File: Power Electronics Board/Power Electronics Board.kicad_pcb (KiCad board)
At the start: 2 copper layers, 137.7 x 71.1 mm, 69 parts, among them J1 Conn_01x02, J2 Conn_01x02, J3 1054301102, J4 1054301102, J5 1054311102, J6 Conn_01x02, J7 1054301108, K2 AZ2150-1A-12DEF, K3 EW60-1A3-CL12D04,00000, K4 DS1E-ML-DC12V, Q1 AO3400A, Q2 AO3400A, Q3 DMG2301L, U1 MCP6004, U3 MCP1703AT-5002E/CB, U4 CC1R5-1205SR-E, U5 ISOM8111DFSR, U6 MCP6004, U7 LM555xM, U8 SZNUD3124LT1G

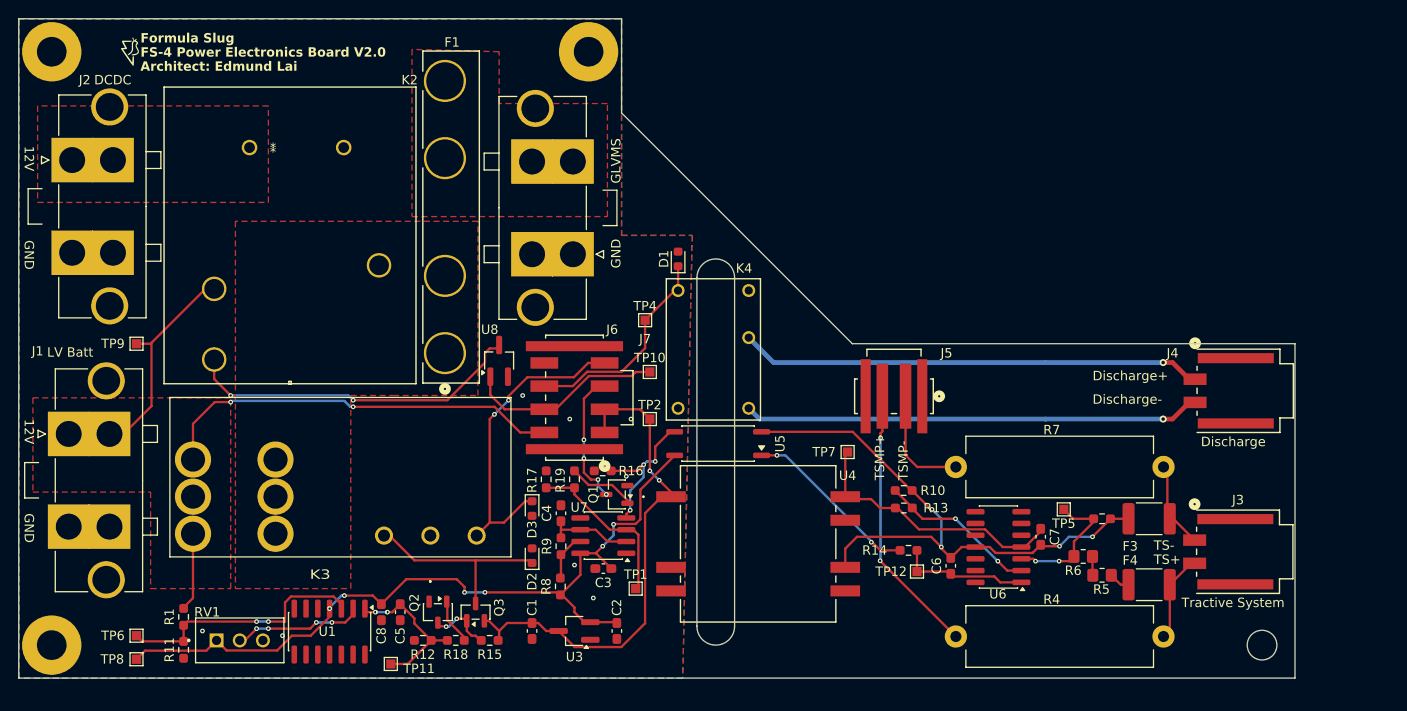
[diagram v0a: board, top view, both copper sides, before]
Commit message: Rev 2.52
Changed DCDC Connector into studs to save vertical space
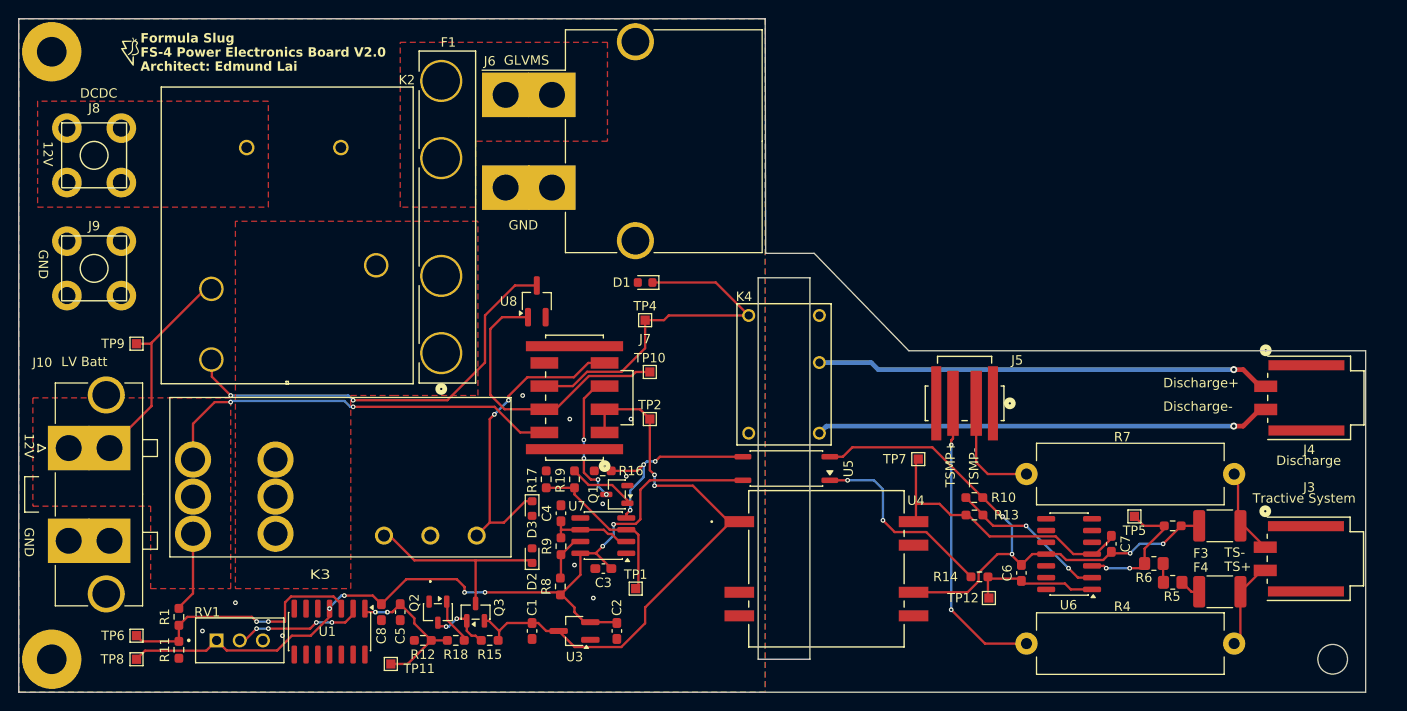
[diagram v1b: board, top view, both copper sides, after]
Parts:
- removed H5: MountingHole_Pad, MountingHole:MountingHole_3.2mm_M3_Pad
- removed J1, J2: Conn_01x02, FS_4_Global_Footprint_Library:Molex_Mini-Fit_Sr_42819-22XX_1x02_P10.00mm_Vertical
- added J10: Conn_01x02, FS_4_Global_Footprint_Library:Molex_Mini-Fit_Sr_42819-22XX_1x02_P10.00mm_Vertical, F.Cu at (54.2, 123.5)
- added J8: 74651173R, FS_4_Global_Footprint_Library:74651173R, F.Cu at (56.9, 91.9)
- added J9: 74651173R, FS_4_Global_Footprint_Library:74651173R, F.Cu at (56.9, 104.1)
- J6: footprint FS_4_Global_Footprint_Library:Molex_Mini-Fit_Sr_42819-22XX_1x02_P10.00mm_Vertical -> FS_4_Global_Footprint_Library:Molex_Mini-Fit_Sr_42820-22XX_1x02_P10.00mm_Horizontal
- moved J6 18.7 mm to (101.3, 85.4), turned to 0 degrees
- moved TP12 8.27 mm to (153.4, 139.7)
- moved R14 8.17 mm to (152.4, 137.4)
- moved K4 8.08 mm to (127.5, 109.2)
- moved U5 7.84 mm to (131.6, 125.7)
- moved U4 7.84 mm to (135.9, 136.5)
- moved H3 7.77 mm to (190.5, 146.3)
- moved C6 7.66 mm to (156.9, 137.0)
- moved C7 7.66 mm to (166.6, 133.9)
- moved F3 7.66 mm to (178.3, 131.9)
- moved F4 7.66 mm to (178.3, 139.0)
- moved J3 7.66 mm to (187.9, 135.5)
- moved J4 7.66 mm to (188.0, 118.1)
- moved R13 7.66 mm to (151.9, 130.7)
- moved R2 7.66 mm to (173.2, 131.9)
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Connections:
- J6 pad 1: GND -> GLVMS
- J6 pad 2: GLVMS -> GND
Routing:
- net Shutdown_Final: track 23.3 -> 38.8 mm
- net TS_Ready: track 21.5 -> 31.2 mm
- net Net-(K2-Pad3): track 36.7 -> 46.2 mm
- net +12V_Switched: track 54.0 -> 62.2 mm
- net +5V_LV: track 85.1 -> 91.4 mm
- net Net-(U7-R): track 16.0 -> 21.4 mm
- net Net-(J5-Pin_2): track 29.4 -> 32.0 mm
- net Net-(R14-Pad2): track 19.2 -> 21.5 mm
- net +5V_Isolated: track 29.3 -> 31.5 mm
- net Net-(J4-Pin_1): track 50.2 -> 49.4 mm
- net GND: vias 8 -> 10
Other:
- board size 137.7 x 71.1 mm -> 145.3 x 72.6 mm
